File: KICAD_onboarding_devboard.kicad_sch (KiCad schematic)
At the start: 19 parts, among them U1 STM32G0B1KETx

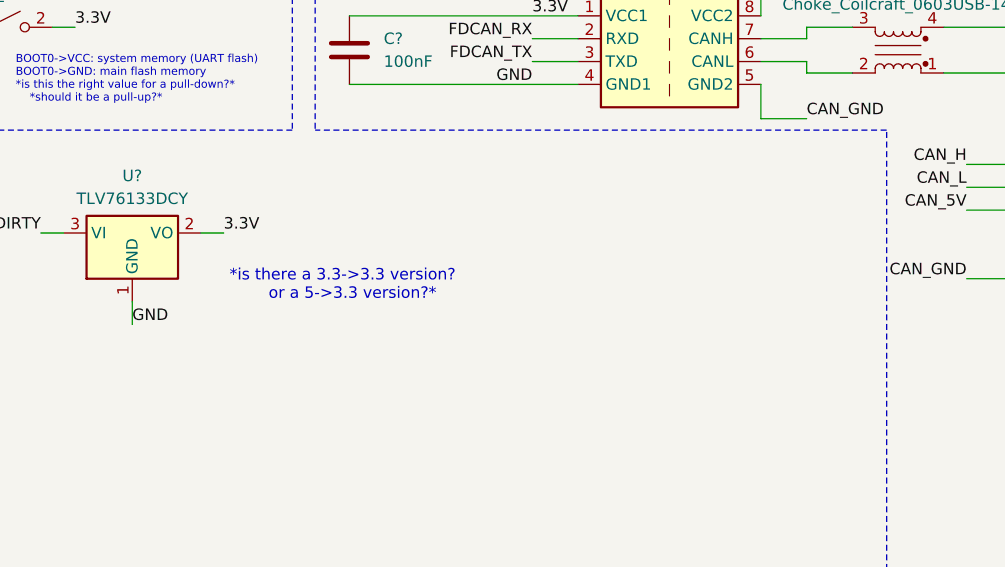
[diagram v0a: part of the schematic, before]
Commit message: br
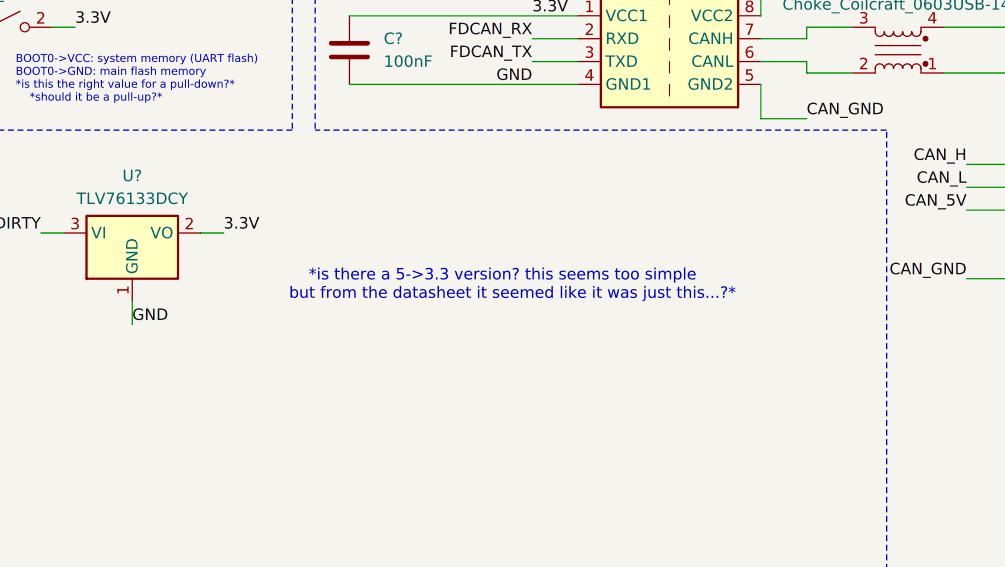
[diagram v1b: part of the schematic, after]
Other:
- note added: "*is there a 5->3.3 version? this seems too simple but from the datasheet it seemed like it was just this...?*"
- note removed: "*is there a 3.3->3.3 version? or a 5->3.3 version?*"
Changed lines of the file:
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@@
 		)
 	)
-	(text "*is there a 3.3->3.3 version? \n	or a 5->3.3 version?*"
+	(text "*is there a 5->3.3 version? this seems too simple\n	but from the datasheet it seemed like it was just this...?*"
 		(exclude_from_sim no)
-		(at 174.498 62.992 0)
+		(at 192.278 62.992 0)
 		(effects
 			(font
